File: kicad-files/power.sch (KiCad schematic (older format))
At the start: 38 parts

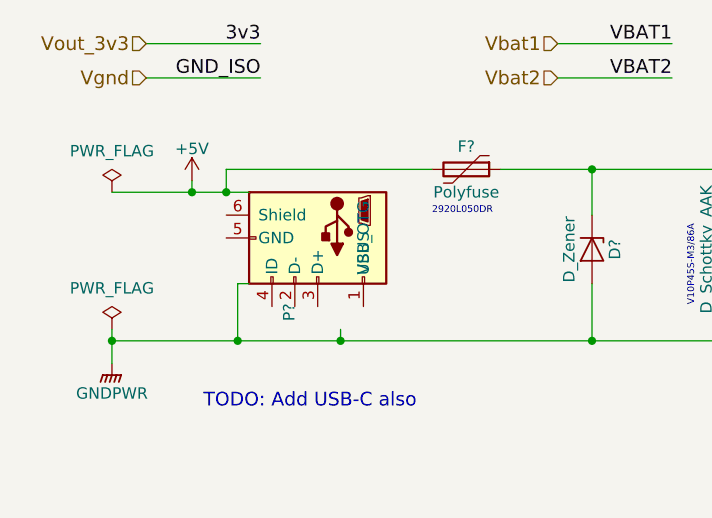
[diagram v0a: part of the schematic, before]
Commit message: kicad-4.0.7
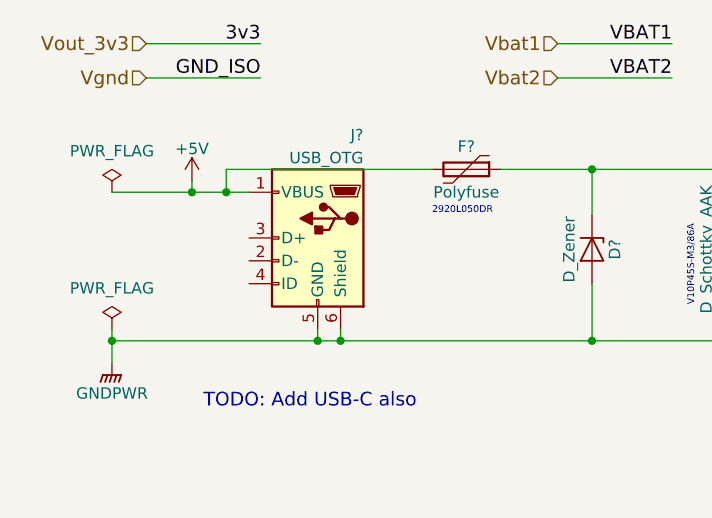
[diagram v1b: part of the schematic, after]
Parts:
- removed P?: USB_OTG, symbol USB_OTG
- added J?: USB_OTG, symbol USB_OTG
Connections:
- net +5V: now also J?.1 (VBUS)
- net GNDPWR: now also J?.5 (GND), J?.6 (Shield)
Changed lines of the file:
@@
 EESchema Schematic File Version 2
+LIBS:OpenHardwareHolterMonitor-rescue
 LIBS:power
 LIBS:device
@@
 VBAT2
 $Comp
-L USB_OTG P?
-U 1 1 5AAD4608
-P 1800 1500
-F 0 "P?" H 2125 1375 50  0000 C CNN
-F 1 "USB_OTG" H 1800 1700 50  0000 C CNN
-F 2 "" V 1750 1400 50  0000 C CNN
-F 3 "" V 1750 1400 50  0000 C CNN
-	1    1800 1500
-	0    1    1    0
-$EndComp
-$Comp
 L GNDPWR #PWR?
 U 1 1 5AAD4720
@@
 	900  1950 4650 1950
 Wire Wire Line
-	1450 1950 1450 1700
-Wire Wire Line
-	1450 1700 1500 1700
-Wire Wire Line
 	900  1300 1500 1300
 Wire Wire Line
 	1250 1300 1250 1250
 Connection ~ 1250 1300
-Connection ~ 1450 1950
 Wire Wire Line
 	1900 1950 1900 1900
@@
 Text Notes 9500 2100 0    60   ~ 0
 Optional Power Indicator
+$Comp
+L USB_OTG J?
+U 1 1 5AD33DB1
+P 1800 1500
+F 0 "J?" H 1600 1950 50  0000 L CNN
+F 1 "USB_OTG" H 1600 1850 50  0000 L CNN
+F 2 "" H 1950 1450 50  0001 C CNN
+F 3 "" H 1950 1450 50  0001 C CNN
+	1    1800 1500
+	-1   0    0    -1
+$EndComp
+Wire Wire Line
+	1800 1900 1800 1950
+Connection ~ 1800 1950
 $EndSCHEMATC
